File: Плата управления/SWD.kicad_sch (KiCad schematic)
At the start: 2 parts, among them J10 SWD

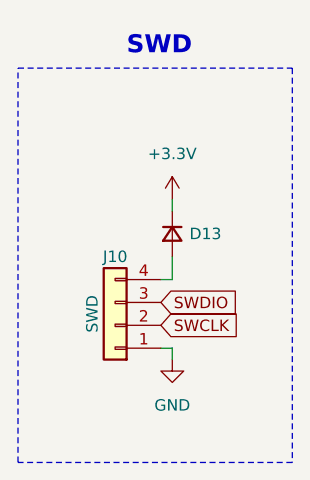
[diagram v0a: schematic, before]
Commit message: Версия под отчёт
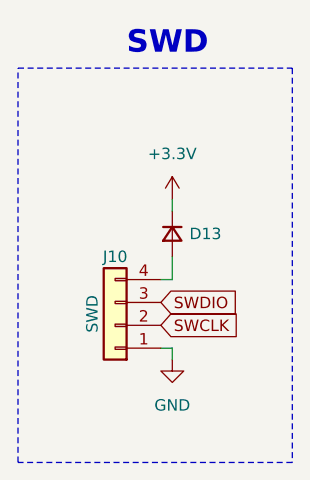
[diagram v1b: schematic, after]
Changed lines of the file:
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@@
   )
   (text "SWD" (at 153.035 78.105 0)
-    (effects (font (size 2 2) bold) (justify left bottom))
+    (effects (font (size 2.5 2.5) bold) (justify left bottom))
   )
   (global_label "SWCLK" (shape input) (at 156.845 107.95 0) (fields_autoplaced)
@@
           (reference "#PWR0105") (unit 1)
         )
+        (path "/75f4c67c-bbde-4446-8f82-67797a1b269f/a1fd62e4-a3fa-422c-840b-ff6e9353e9fd"
+          (reference "#PWR0110") (unit 1)
+        )
       )
     )
@@
         (path "/75f4c67c-bbde-4446-8f82-67797a1b269f/47f4c3e6-ca16-48bd-a07f-b1f138b5b42e"
           (reference "#PWR0106") (unit 1)
+        )
+        (path "/75f4c67c-bbde-4446-8f82-67797a1b269f/a1fd62e4-a3fa-422c-840b-ff6e9353e9fd"
+          (reference "#PWR0111") (unit 1)
         )
       )
@@
         (path "/75f4c67c-bbde-4446-8f82-67797a1b269f/47f4c3e6-ca16-48bd-a07f-b1f138b5b42e"
           (reference "J10") (unit 1)
+        )
+        (path "/75f4c67c-bbde-4446-8f82-67797a1b269f/a1fd62e4-a3fa-422c-840b-ff6e9353e9fd"
+          (reference "J11") (unit 1)
         )
       )
@@
           (reference "D13") (unit 1)
         )
+        (path "/75f4c67c-bbde-4446-8f82-67797a1b269f/a1fd62e4-a3fa-422c-840b-ff6e9353e9fd"
+          (reference "D16") (unit 1)
+        )
       )
